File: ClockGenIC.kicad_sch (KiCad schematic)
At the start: 24 parts, among them J4 Conn_Coaxial, J5 Conn_Coaxial, J6 Conn_Coaxial, U1 ADF4351, U2 AP2112K-3.3, Y2 TG2520SMN-xx.xxxxxxMhz-xxxxNM

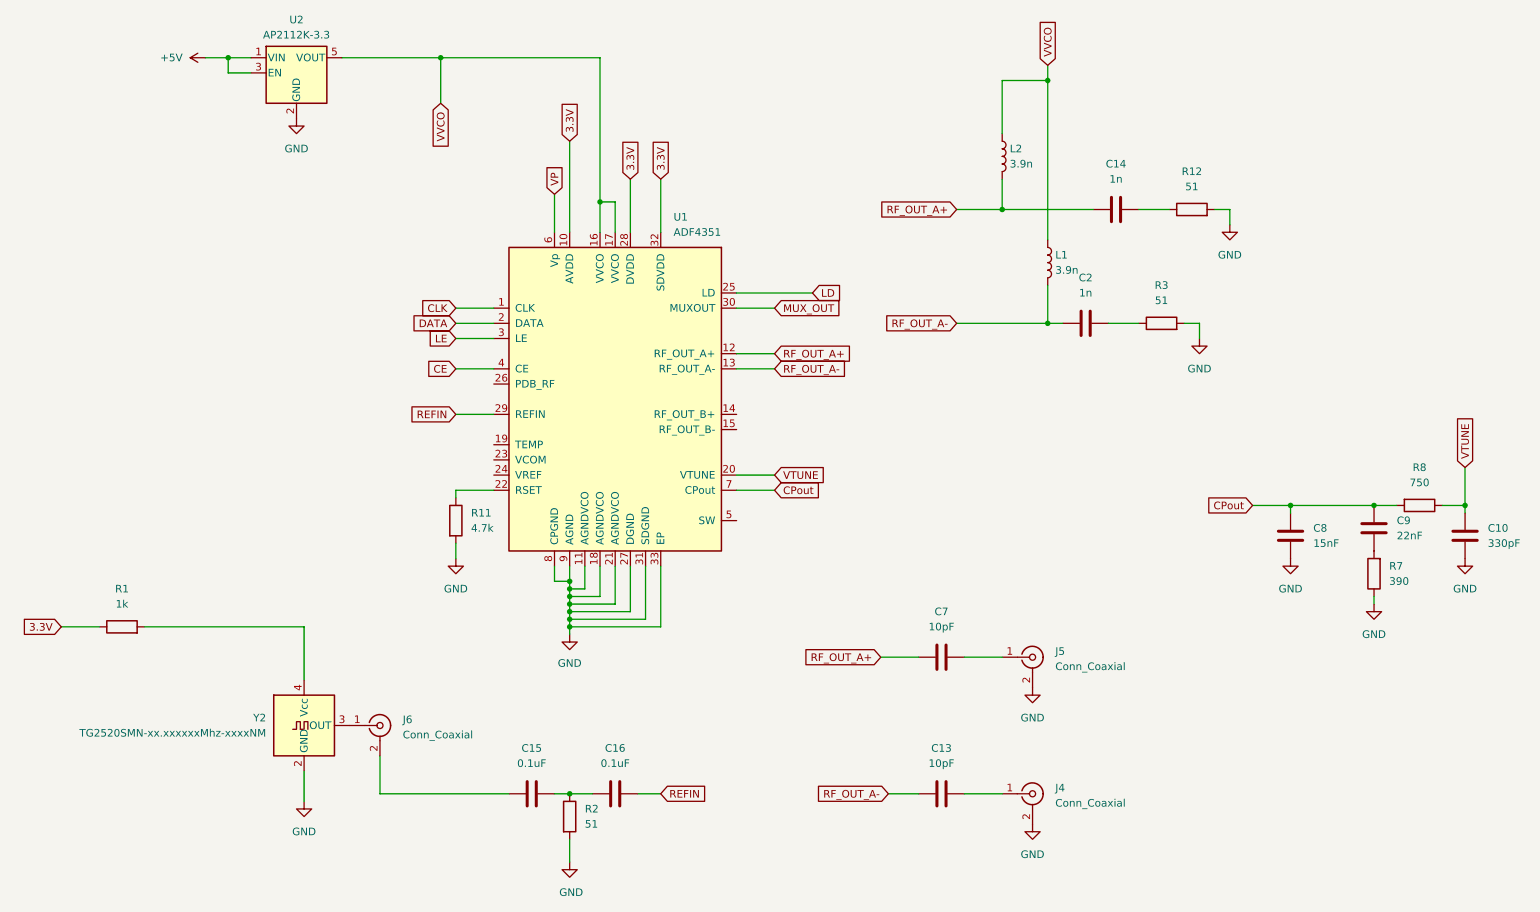
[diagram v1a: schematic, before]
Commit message: Update
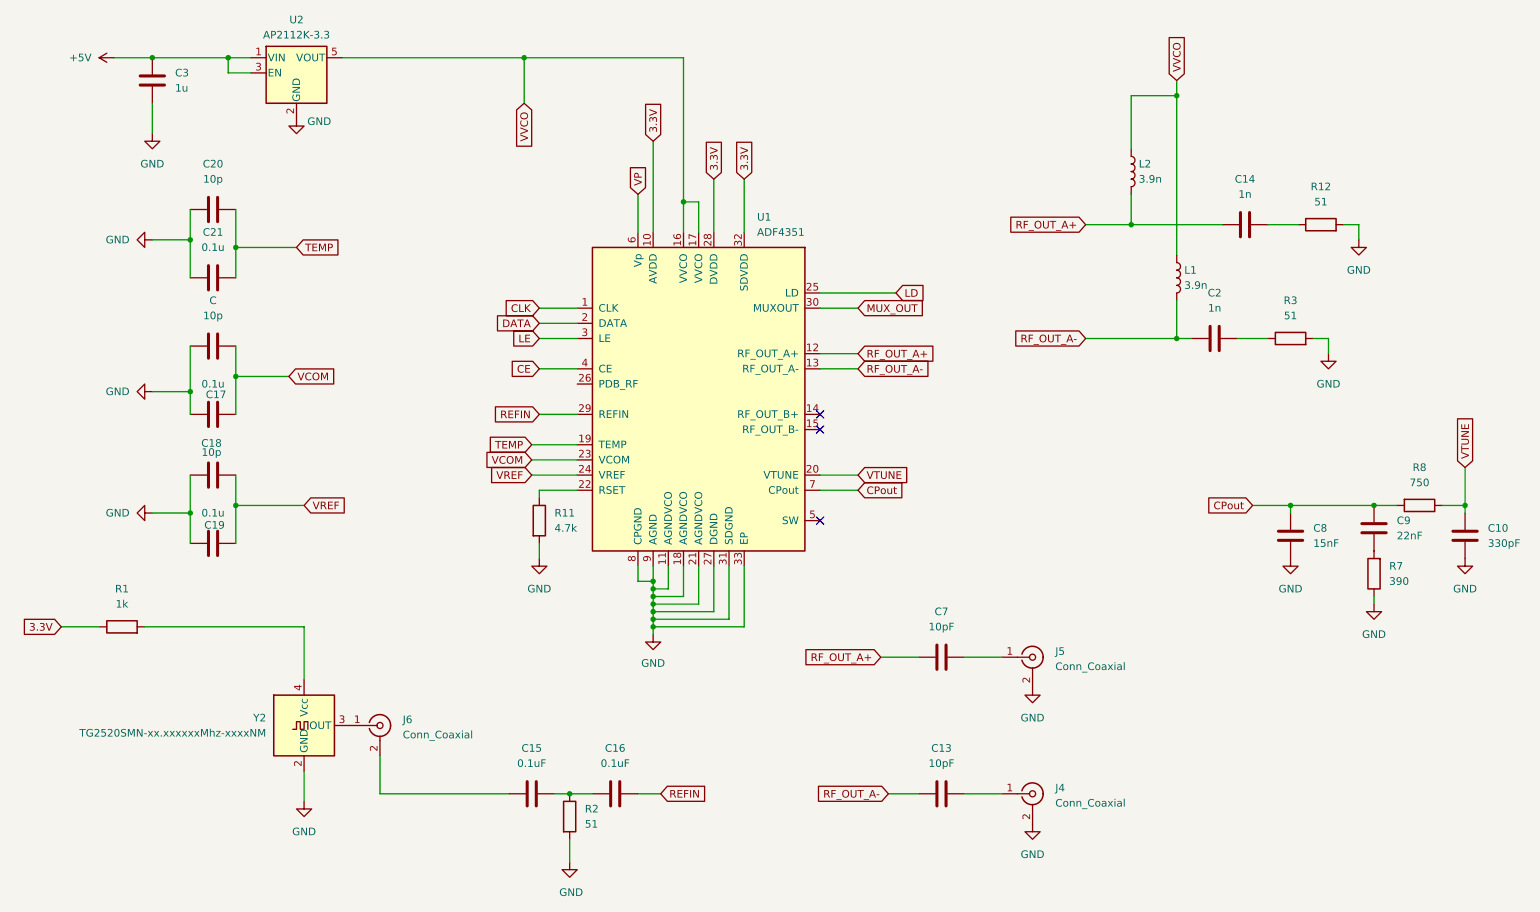
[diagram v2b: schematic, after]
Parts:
- added C, C18, C20: 10p, symbol Device:C
- added C17, C19, C21: 0.1u, symbol Device:C
- added C3: 1u, symbol Device:C
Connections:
- net +5V: now also C3.1
- net GND: now also C.1, C17.1, C18.1, C19.1, C20.1, C21.1, C3.2
- net TEMP: now reaches U1.19 (TEMP)
- net TEMP: now also C20.2, C21.2
- net VCOM: now reaches U1.23 (VCOM)
- net VCOM: now also C.2, C17.2
- net VREF: now reaches U1.24 (VREF)
- net VREF: now also C18.2, C19.2
- no-connect marks 0 -> 3
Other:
- moved on the sheet: C14, C2, L1, L2, R11, R12, R3, U1
